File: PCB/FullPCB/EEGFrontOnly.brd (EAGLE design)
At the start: 87.5 x 90.9 mm, 209 parts, among them IC1 ADS1299-X, IC2 ADUM4160BRWZ, J11 MICRO-SD_CARD_SOCKET, J12 455-1750-1-ND, J13 455-1750-1-ND, J14 455-1750-1-ND, J15 455-1750-1-ND, J2 USB_B_PTH, J8 JTAG, U1 LP2985-33DBVT, U10 HT7318, U11 TMS320F28335PGFA, U12 HT7333, U13 2.93V, U14 MAX811-812, U2 B0505S-1WB0505S-1W, U3 TPS60403DBVT, U4 TPS73225DBVR, U5 TPS73225DBVR, U6 TPD4E1B06DCKR, U7 TPD4E1B06DCKR, U8 TPD4E1B06DCKR, U9 HT7333, Y1 30MHz, Y2 12MHz

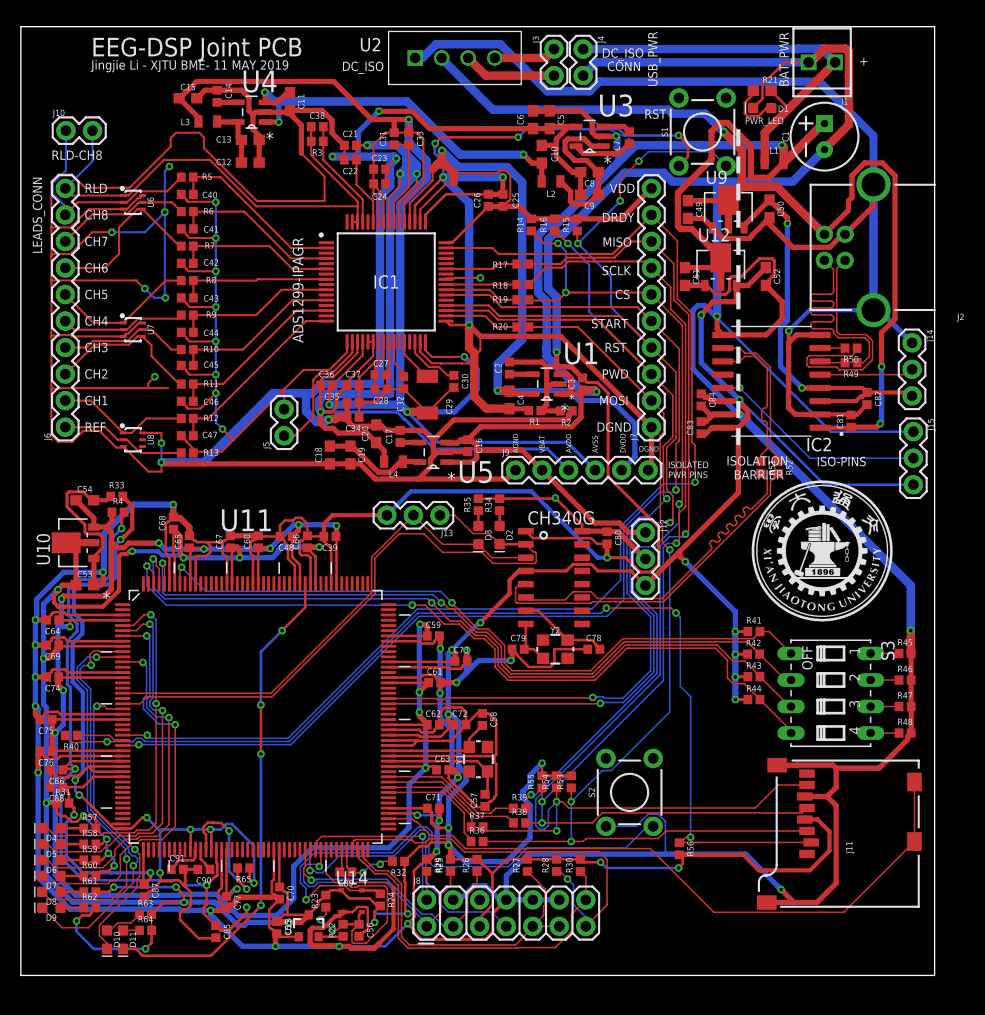
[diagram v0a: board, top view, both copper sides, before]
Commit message: full pcb nearly complete
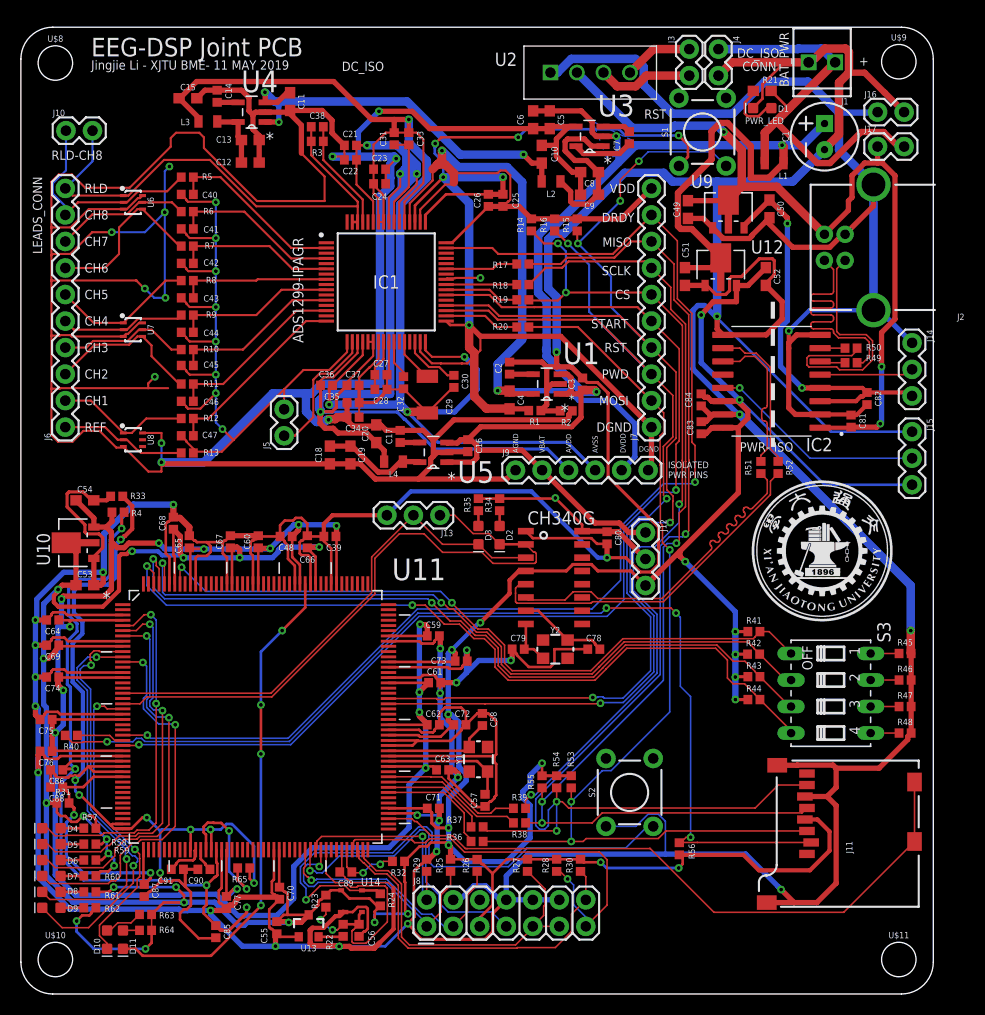
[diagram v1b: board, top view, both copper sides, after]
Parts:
- added J16, J17: (no value), SparkFun-Connectors:1X02
- added U$10, U$11, U$8, U$9: (no value), SparkFun-Hardware:STAND-OFF
- moved U2 13.0 mm to (51.0, 86.6)
- moved J3 13.0 mm to (64.3, 88.8)
- moved J4 13.0 mm to (67.1, 88.8)
- moved J15 0.13 mm to (85.6, 52.2)
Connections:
- net GND: now also J16.2
- net GND-ISO: now also J16.1
- net VBATPRE: now also J17.2
- net VCC-ISO: now also J17.1
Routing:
- net VCC-ISO: track 95.8 -> 84.0 mm
- net GND-ISO: track 123.3 -> 115.7 mm
- net GND: track 789.5 -> 783.1 mm
- net VBATPRE: track 39.6 -> 42.3 mm
- net N$1: track 6.03 -> 6.61 mm
- net VBAT: track 146.0 -> 145.5 mm
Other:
- board size 87.5 x 90.9 mm -> 87.4 x 92.6 mm
- board text added: "PWR- ISO"
- board text removed: "ISO-PINS"
- board text removed: "ISOLATION BARRIER"
- board text removed: "USB_PWR"
